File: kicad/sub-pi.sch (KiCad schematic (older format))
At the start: 23 parts, among them J2 RPI, Q1 AO3404 (Q_NMOS_GSD), Q2 AO3404 (Q_NMOS_GSD), U3 NCP1117-5.0_TO252, U4 NCP1117-3.3_TO252, U5 NCP1117-5.0_TO252, U6 NCP1117-3.3_TO252, U7 SI9933ADY, U8 LTC1154

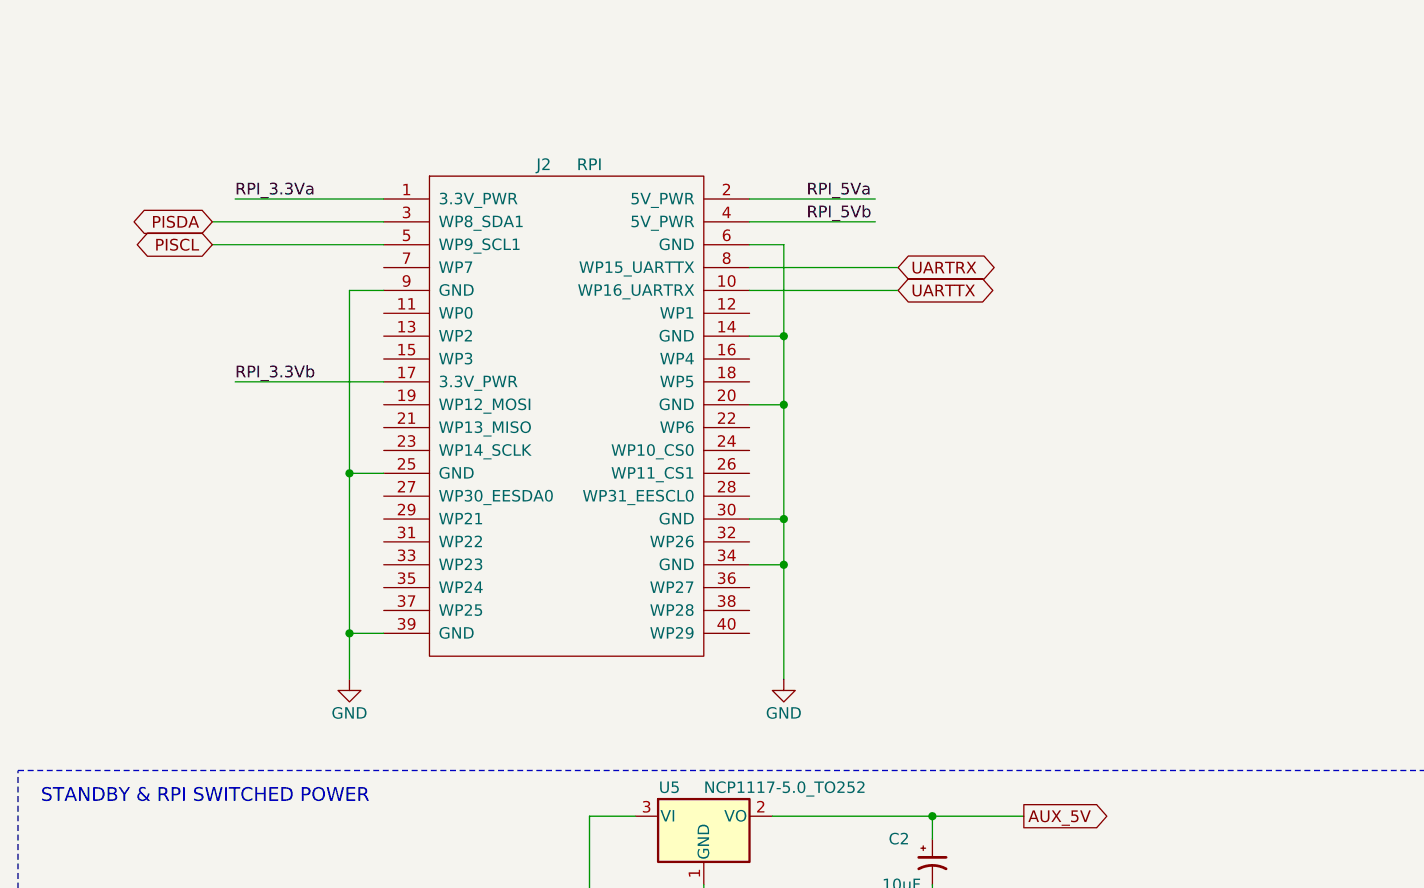
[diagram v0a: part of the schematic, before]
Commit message: Media migration.
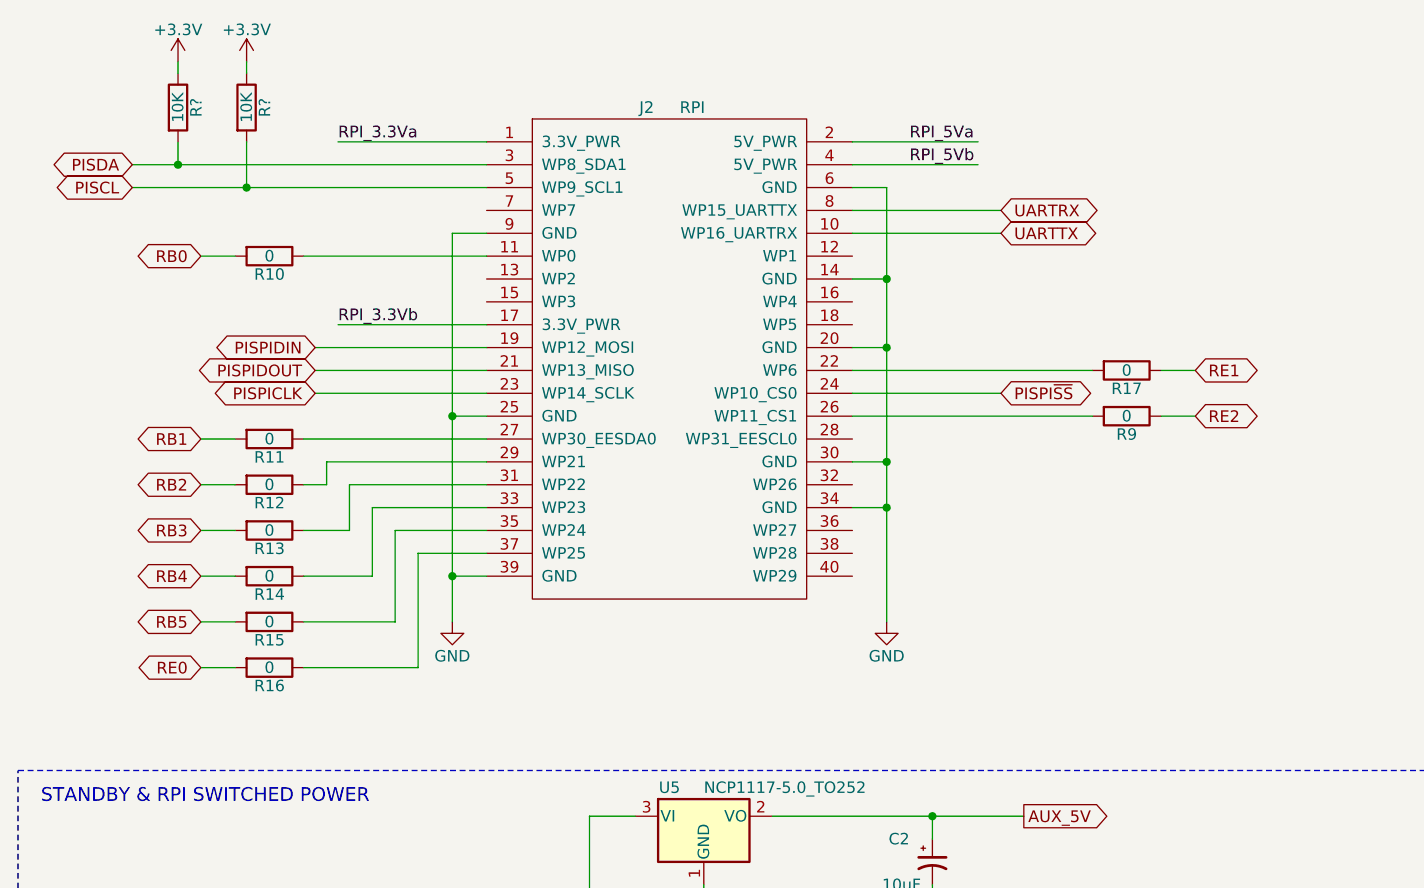
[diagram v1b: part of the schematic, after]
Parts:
- added R10, R11, R12, R13, R14, R15, R16, R17, R9: 0, symbol R
- added R? (x2): 10K, symbol R
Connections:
- net labels added: +3.3V, PISPICLK, PISPIDIN, PISPIDOUT, PISPI~SS~, RB0, RB1, RB2, RB3, RB4, RB5, RE0, RE1, RE2
- wire segments 98 -> 134
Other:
- moved on the sheet: J2
